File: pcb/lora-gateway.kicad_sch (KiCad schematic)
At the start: 13 parts, among them J1 USB_B_Micro, J2 Conn_01x06, J3 Conn_01x06, J4 Conn_Coaxial, J5 AVR-JTAG-10, J6 AVR-ISP-6, U1 RFM95W-868S2, U2 ATmega2560-16A, U3 LM1117-3.3

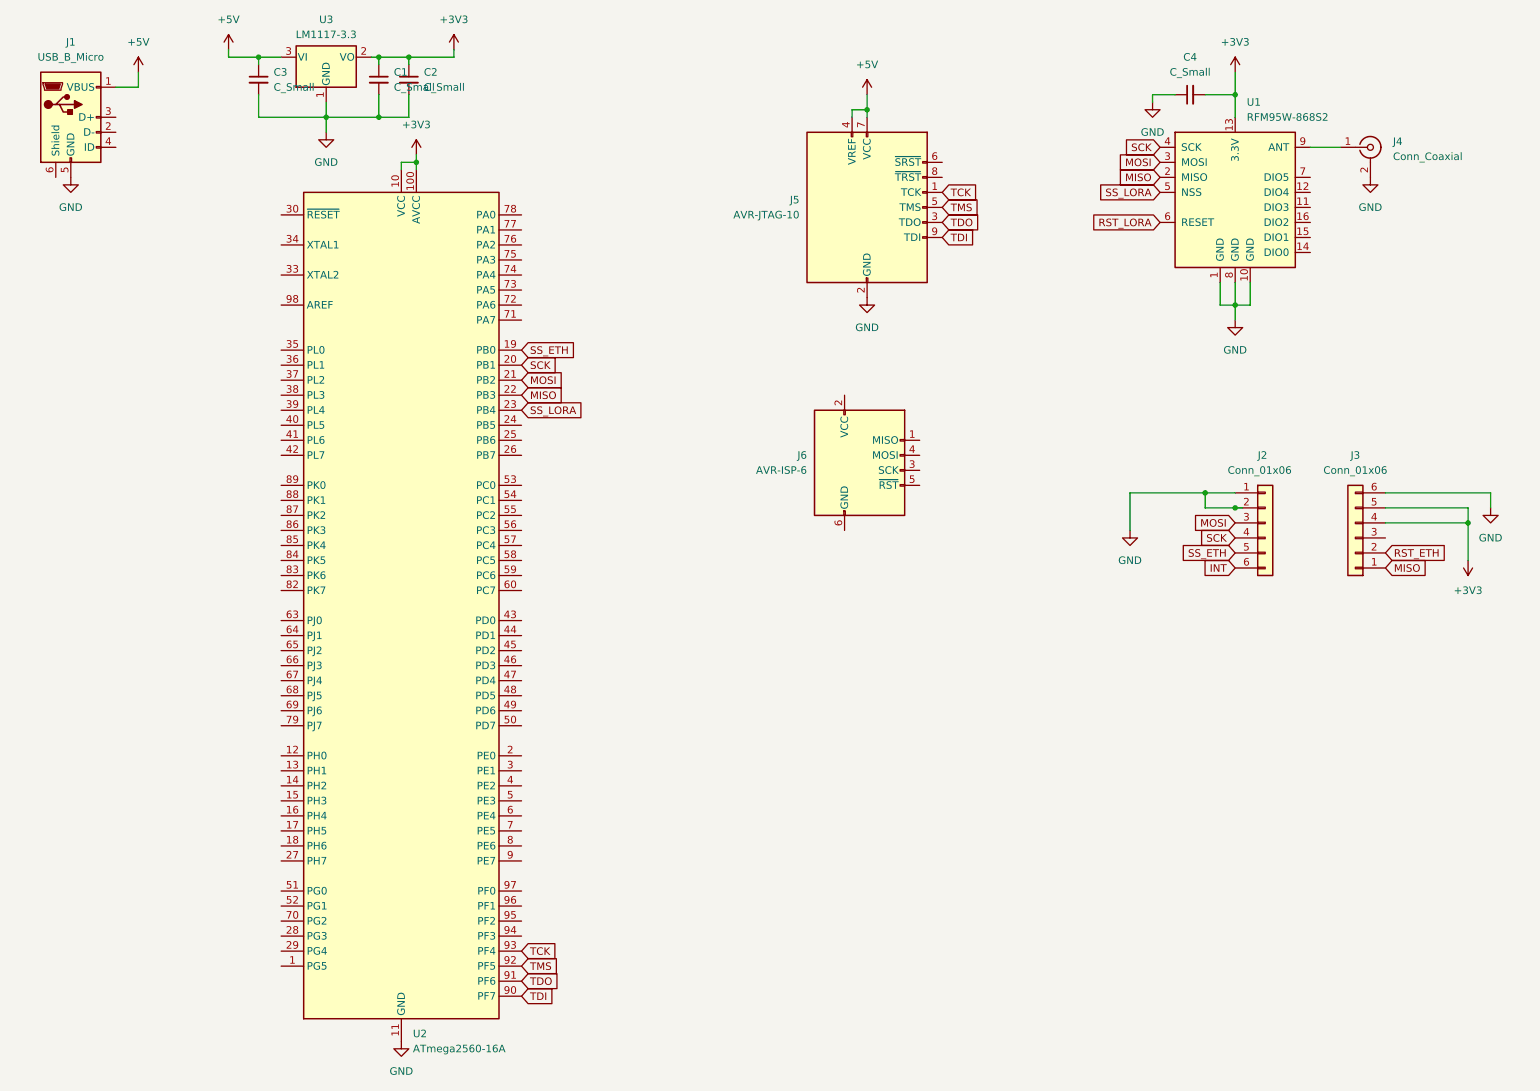
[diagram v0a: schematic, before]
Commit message: pcb wiring
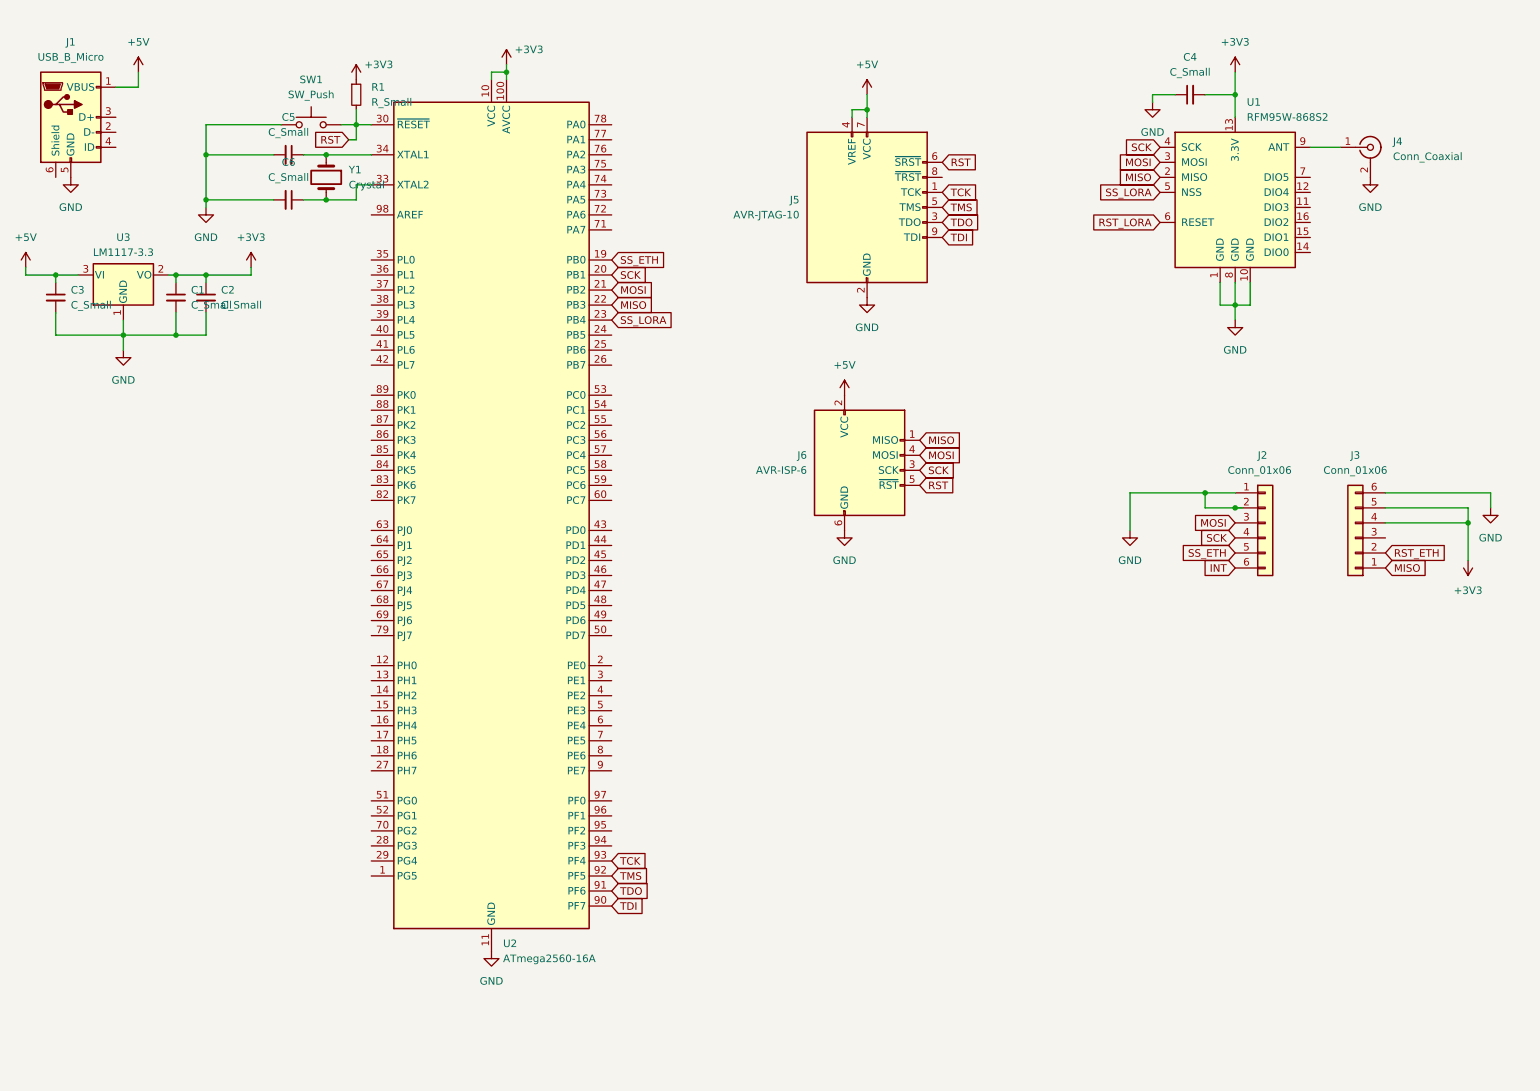
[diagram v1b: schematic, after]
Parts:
- added C5, C6: C_Small, Capacitor_SMD:C_0603_1608Metric, symbol Device:C_Small
- added R1: R_Small, Resistor_SMD:R_0603_1608Metric, symbol Device:R_Small
- added SW1: SW_Push, Button_Switch_SMD:SW_SPST_CK_RS282G05A3, symbol Switch:SW_Push
- added Y1: Crystal, Crystal:Crystal_SMD_5032-2Pin_5.0x3.2mm, symbol Device:Crystal
- J5: footprint (none) -> Connector_PinHeader_2.54mm:PinHeader_2x05_P2.54mm_Vertical
- J6: footprint (none) -> Connector_PinHeader_2.54mm:PinHeader_2x03_P2.54mm_Vertical
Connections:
- net +3V3: now also R1.1
- net +5V: now also J6.2 (VCC)
- net GND: now also J6.6 (GND), C5.2, C6.2, SW1.1
- net MISO: now also J6.1 (MISO)
- net MOSI: now also J6.4 (MOSI)
- net SCK: now also J6.3 (SCK)
- net RST: now reaches U2.30 (~{RESET})
- net RST: now also J5.6 (~{SRST}), J6.5 (~{RST}), R1.2, SW1.2
- net at U2.33 (XTAL2): now also C6.1, Y1.2
- net at U2.34 (XTAL1): now also C5.1, Y1.1
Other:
- moved on the sheet: C1, C2, C3, U2, U3

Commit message: up schematic
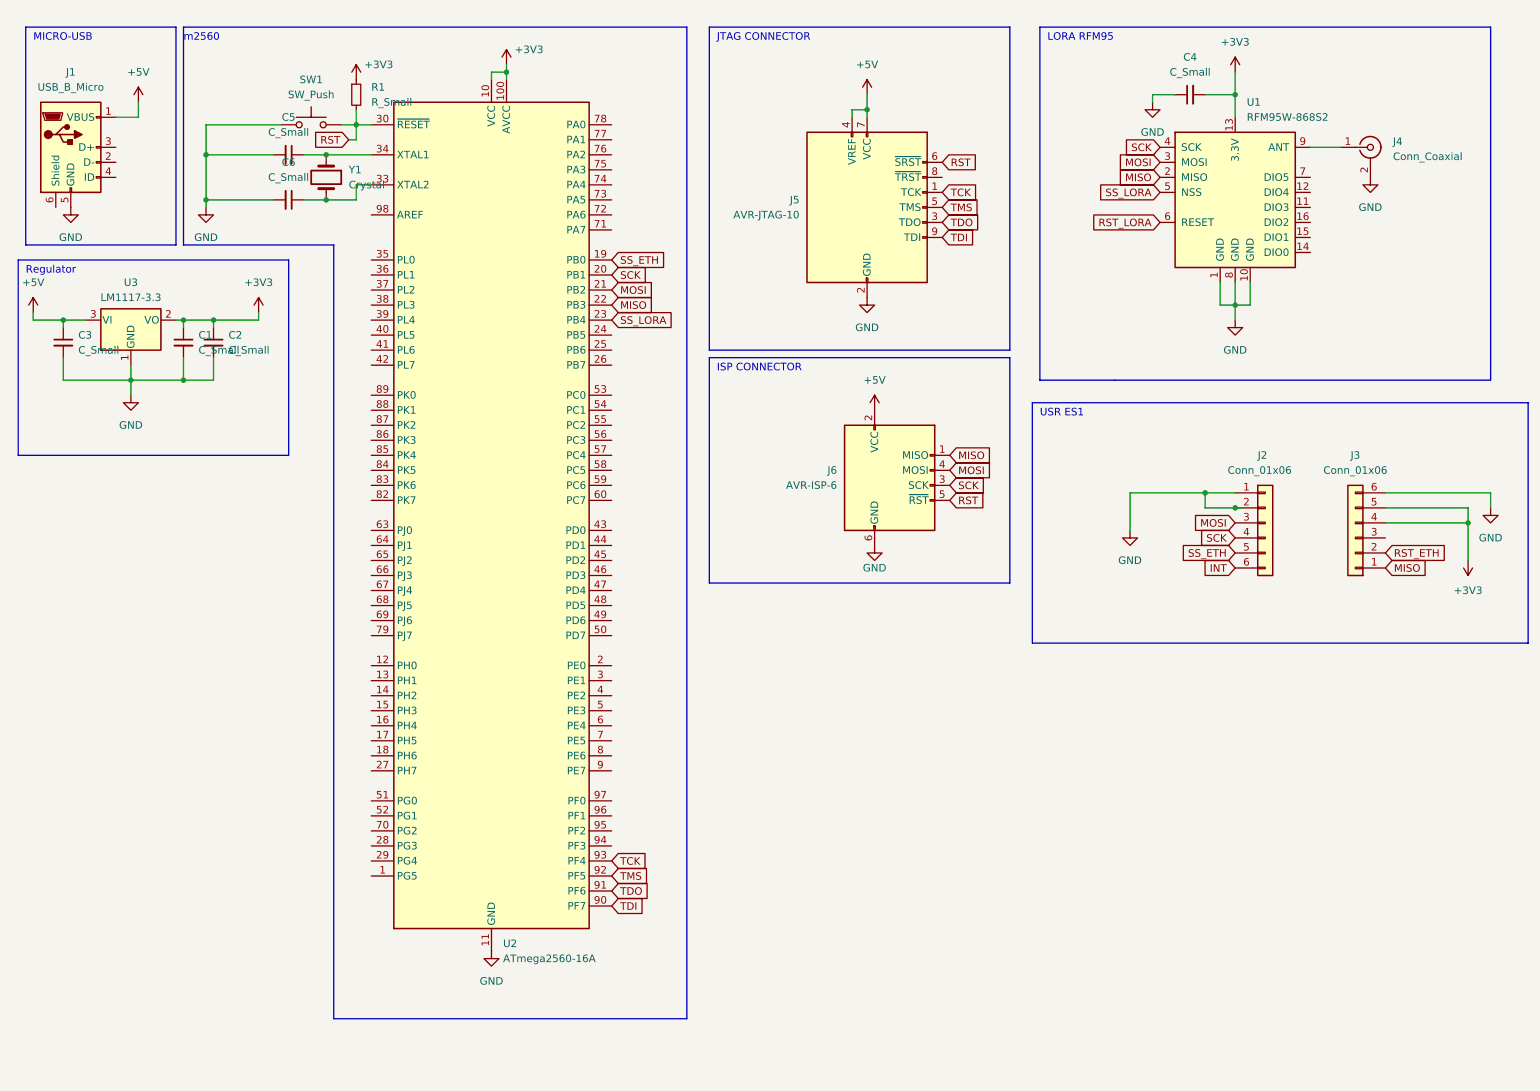
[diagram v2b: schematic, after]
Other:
- note added: "ISP CONNECTOR"
- note added: "JTAG CONNECTOR"
- note added: "LORA RFM95"
- note added: "MICRO-USB"
- note added: "Regulator"
- note added: "USR ES1"
- note added: "m2560"
- moved on the sheet: C1, C2, C3, J1, J6, U3
